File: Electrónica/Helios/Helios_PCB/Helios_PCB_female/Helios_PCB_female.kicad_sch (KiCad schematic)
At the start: 8 parts, among them J1 Conn_01x02_Socket, J2 Conn_01x02_Socket, J3 Conn_01x02_Socket, J4 Conn_01x02_Socket, J7 Conn_01x02_Socket

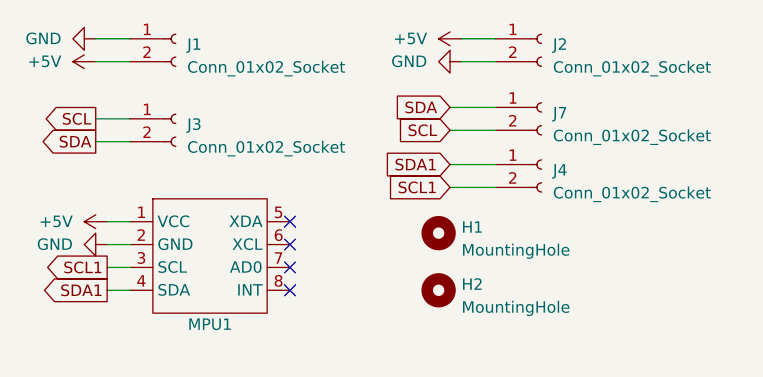
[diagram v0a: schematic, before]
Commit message: V2.2 - BNO_055 IMU
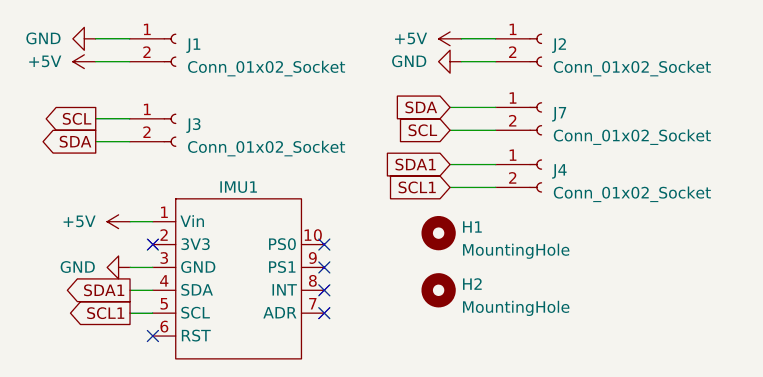
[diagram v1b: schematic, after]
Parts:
- removed MPU1: ~, MPU6050:MPU6050_module, symbol MPU6050:MPU6050
- added IMU1: ~, BNO_055:BNO_055, symbol BNO_055:BNO_055
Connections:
- net +5V: now also IMU1.1 (Vin)
- net GND: now also IMU1.3 (GND)
- net SCL1: now also IMU1.5 (SCL)
- net SDA1: now also IMU1.4 (SDA)
- no-connect marks 4 -> 6
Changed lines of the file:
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@@
 (kicad_sch (version 20230121) (generator eeschema)
   (paper "A4")
-  (no_connect (at 143.51 105.41))
-  (no_connect (at 143.51 107.95))
-  (no_connect (at 143.51 113.03))
-  (no_connect (at 143.51 110.49))
+  (no_connect (at 147.32 107.95))
+  (no_connect (at 147.32 110.49))
+  (no_connect (at 128.27 118.11))
+  (no_connect (at 147.32 115.57))
+  (no_connect (at 147.32 113.03))
+  (no_connect (at 128.27 107.95))
   (wire (pts (xy 121.92 96.52) (xy 125.73 96.52))
     (stroke (width 0) (type default))
   )
-  (wire (pts (xy 125.73 105.41) (xy 123.19 105.41))
+  (wire (pts (xy 128.27 105.41) (xy 125.73 105.41))
     (stroke (width 0) (type default))
   )
@@
     (stroke (width 0) (type default))
   )
-  (wire (pts (xy 123.19 110.49) (xy 125.73 110.49))
+  (wire (pts (xy 125.73 115.57) (xy 128.27 115.57))
     (stroke (width 0) (type default))
   )
@@
     (stroke (width 0) (type default))
   )
-  (wire (pts (xy 123.19 113.03) (xy 125.73 113.03))
-    (stroke (width 0) (type default))
-  )
-  (wire (pts (xy 123.19 107.95) (xy 125.73 107.95))
+  (wire (pts (xy 125.73 113.03) (xy 128.27 113.03))
+    (stroke (width 0) (type default))
+  )
+  (wire (pts (xy 125.73 110.49) (xy 128.27 110.49))
     (stroke (width 0) (type default))
   )
@@
     (stroke (width 0) (type default))
   )
-  (global_label "SCL1" (shape output) (at 123.19 110.49 180) (fields_autoplaced)
-    (effects (font (size 1.27 1.27)) (justify right))
-    (property "Intersheetrefs" "${INTERSHEET_REFS}" (at 115.5671 110.49 0)
+  (global_label "SCL1" (shape output) (at 125.73 115.57 180) (fields_autoplaced)
+    (effects (font (size 1.27 1.27)) (justify right))
+    (property "Intersheetrefs" "${INTERSHEET_REFS}" (at 118.1071 115.57 0)
       (effects (font (size 1.27 1.27)) (justify right) hide)
     )
@@
     )
   )
-  (global_label "SDA1" (shape output) (at 123.19 113.03 180) (fields_autoplaced)
-    (effects (font (size 1.27 1.27)) (justify right))
-    (property "Intersheetrefs" "${INTERSHEET_REFS}" (at 115.5066 113.03 0)
+  (global_label "SDA1" (shape output) (at 125.73 113.03 180) (fields_autoplaced)
+    (effects (font (size 1.27 1.27)) (justify right))
+    (property "Intersheetrefs" "${INTERSHEET_REFS}" (at 118.0466 113.03 0)
       (effects (font (size 1.27 1.27)) (justify right) hide)
     )
@@
     )
   )
-  (symbol (lib_id "MPU6050:MPU6050") (at 134.62 109.22 0) (unit 1)
-    (in_bom yes) (on_board yes) (dnp no)
-    (property "Reference" "MPU1" (at 134.62 116.84 0)
+  (symbol (lib_id "power:+5V") (at 121.92 87.63 90) (unit 1)
+    (in_bom yes) (on_board yes) (dnp no)
+    (property "Reference" "#PWR03" (at 125.73 87.63 0)
+      (effects (font (size 1.27 1.27)) hide)
+    )
+    (property "Value" "+5V" (at 118.11 87.63 90)
+      (effects (font (size 1.27 1.27)) (justify left))
+    )
+    (property "Footprint" "" (at 121.92 87.63 0)
+      (effects (font (size 1.27 1.27)) hide)
+    )
+    (property "Datasheet" "" (at 121.92 87.63 0)
+      (effects (font (size 1.27 1.27)) hide)
+    )
+    (pin "1")
+    (instances
+      (project "Helios_PCB_female"
+        (path "/48a2e939-e701-47dd-b50e-977aeeb0d1a3"
+          (reference "#PWR03") (unit 1)
+        )
+      )
+    )
+  )
+  (symbol (lib_id "BNO_055:BNO_055") (at 138.43 111.76 0) (unit 1)
+    (in_bom yes) (on_board yes) (dnp no) (fields_autoplaced)
+    (property "Reference" "IMU1" (at 137.795 101.6 0)
       (effects (font (size 1.27 1.27)))
     )
-    (property "Value" "~" (at 119.38 109.22 0)
+    (property "Value" "~" (at 138.43 111.76 0)
       (effects (font (size 1.27 1.27)))
     )
-    (property "Footprint" "MPU6050:MPU6050_module" (at 119.38 109.22 0)
-      (effects (font (size 1.27 1.27)) hide)
-    )
-    (property "Datasheet" "" (at 119.38 109.22 0)
-      (effects (font (size 1.27 1.27)) hide)
-    )
-    (pin "1")
+    (property "Footprint" "BNO_055:BNO_055" (at 138.43 111.76 0)
+      (effects (font (size 1.27 1.27)) hide)
+    )
+    (property "Datasheet" "" (at 138.43 111.76 0)
+      (effects (font (size 1.27 1.27)) hide)
+    )
+    (pin "1")
+    (pin "10")
     (pin "2")
     (pin "3")
@@
     (pin "7")
     (pin "8")
-    (instances
-      (project "Helios_PCB_female"
-        (path "/48a2e939-e701-47dd-b50e-977aeeb0d1a3"
-          (reference "MPU1") (unit 1)
-        )
-      )
-    )
-  )
-  (symbol (lib_id "power:+5V") (at 121.92 87.63 90) (unit 1)
-    (in_bom yes) (on_board yes) (dnp no)
-    (property "Reference" "#PWR03" (at 125.73 87.63 0)
-      (effects (font (size 1.27 1.27)) hide)
-    )
-    (property "Value" "+5V" (at 118.11 87.63 90)
-      (effects (font (size 1.27 1.27)) (justify left))
-    )
-    (property "Footprint" "" (at 121.92 87.63 0)
-      (effects (font (size 1.27 1.27)) hide)
-    )
-    (property "Datasheet" "" (at 121.92 87.63 0)
-      (effects (font (size 1.27 1.27)) hide)
-    )
-    (pin "1")
-    (instances
-      (project "Helios_PCB_female"
-        (path "/48a2e939-e701-47dd-b50e-977aeeb0d1a3"
-          (reference "#PWR03") (unit 1)
+    (pin "9")
+    (instances
+      (project "Helios_PCB_female"
+        (path "/48a2e939-e701-47dd-b50e-977aeeb0d1a3"
+          (reference "IMU1") (unit 1)
         )
       )
@@
     )
   )
-  (symbol (lib_id "power:GND") (at 123.19 107.95 270) (unit 1)
-    (in_bom yes) (on_board yes) (dnp no)
-    (property "Reference" "#PWR04" (at 116.84 107.95 0)
-      (effects (font (size 1.27 1.27)) hide)
-    )
-    (property "Value" "GND" (at 119.38 107.95 90)
+  (symbol (lib_id "power:GND") (at 125.73 110.49 270) (unit 1)
+    (in_bom yes) (on_board yes) (dnp no)
+    (property "Reference" "#PWR04" (at 119.38 110.49 0)
+      (effects (font (size 1.27 1.27)) hide)
+    )
+    (property "Value" "GND" (at 121.92 110.49 90)
       (effects (font (size 1.27 1.27)) (justify right))
     )
-    (property "Footprint" "" (at 123.19 107.95 0)
-      (effects (font (size 1.27 1.27)) hide)
-    )
-    (property "Datasheet" "" (at 123.19 107.95 0)
+    (property "Footprint" "" (at 125.73 110.49 0)
+      (effects (font (size 1.27 1.27)) hide)
+    )
+    (property "Datasheet" "" (at 125.73 110.49 0)
       (effects (font (size 1.27 1.27)) hide)
     )
@@
     )
   )
-  (symbol (lib_id "power:+5V") (at 123.19 105.41 90) (unit 1)
-    (in_bom yes) (on_board yes) (dnp no)
-    (property "Reference" "#PWR01" (at 127 105.41 0)
-      (effects (font (size 1.27 1.27)) hide)
-    )
-    (property "Value" "+5V" (at 119.38 105.41 90)
-      (effects (font (size 1.27 1.27)) (justify left))
-    )
-    (property "Footprint" "" (at 123.19 105.41 0)
-      (effects (font (size 1.27 1.27)) hide)
-    )
-    (property "Datasheet" "" (at 123.19 105.41 0)
-      (effects (font (size 1.27 1.27)) hide)
-    )
+  (symbol (lib_id "power:+5V") (at 125.73 105.41 90) (unit 1)
+    (in_bom yes) (on_board yes) (dnp no)
+    (property "Reference" "#PWR01" (at 129.54 105.41 0)
+      (effects (font (size 1.27 1.27)) hide)
+    )
+    (property "Value" "+5V" (at 121.92 105.41 90)
+      (effects (font (size 1.27 1.27)) (justify left))
+    )
+    (property "Footprint" "" (at 125.73 105.41 0)
+      (effects (font (size 1.27 1.27)) hide)
+    )
+    (property "Datasheet" "" (at 125.73 105.41 0)
+      (effects (font (size 1.27 1.27)) hide)
+    )
